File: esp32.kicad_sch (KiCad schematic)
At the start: 13 parts, among them J2 Conn_01x05_Pin, Q3 MMBT3904, Q4 MMBT3904, U14 S32K324NHT1MPBST, Y1 ECS-2520MV-xxx-xx

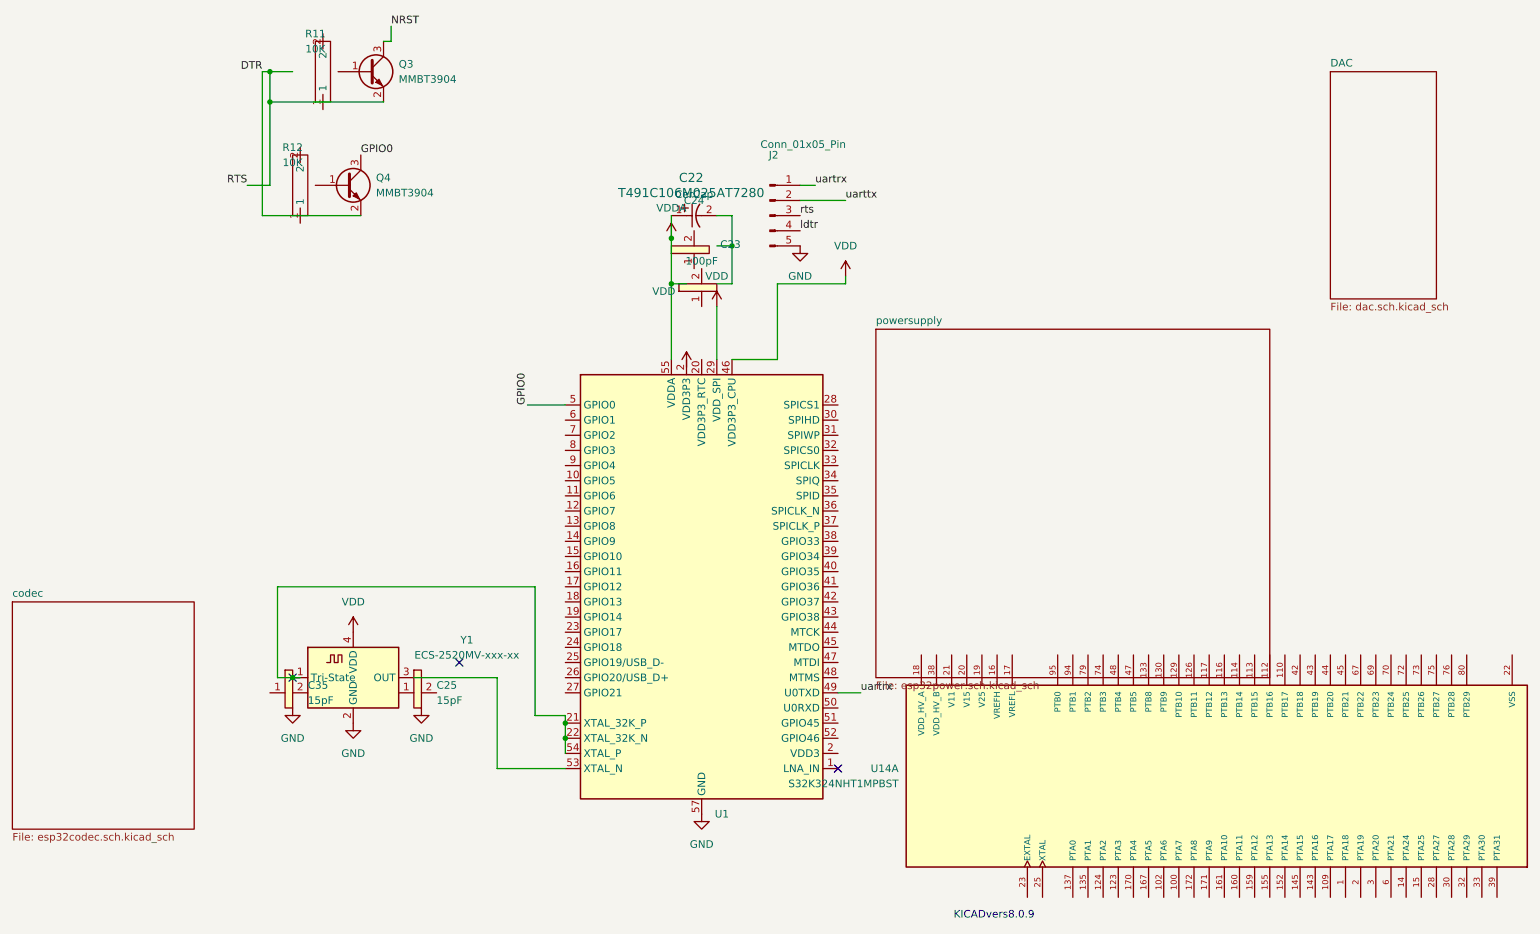
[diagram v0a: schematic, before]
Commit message: recloned first commit
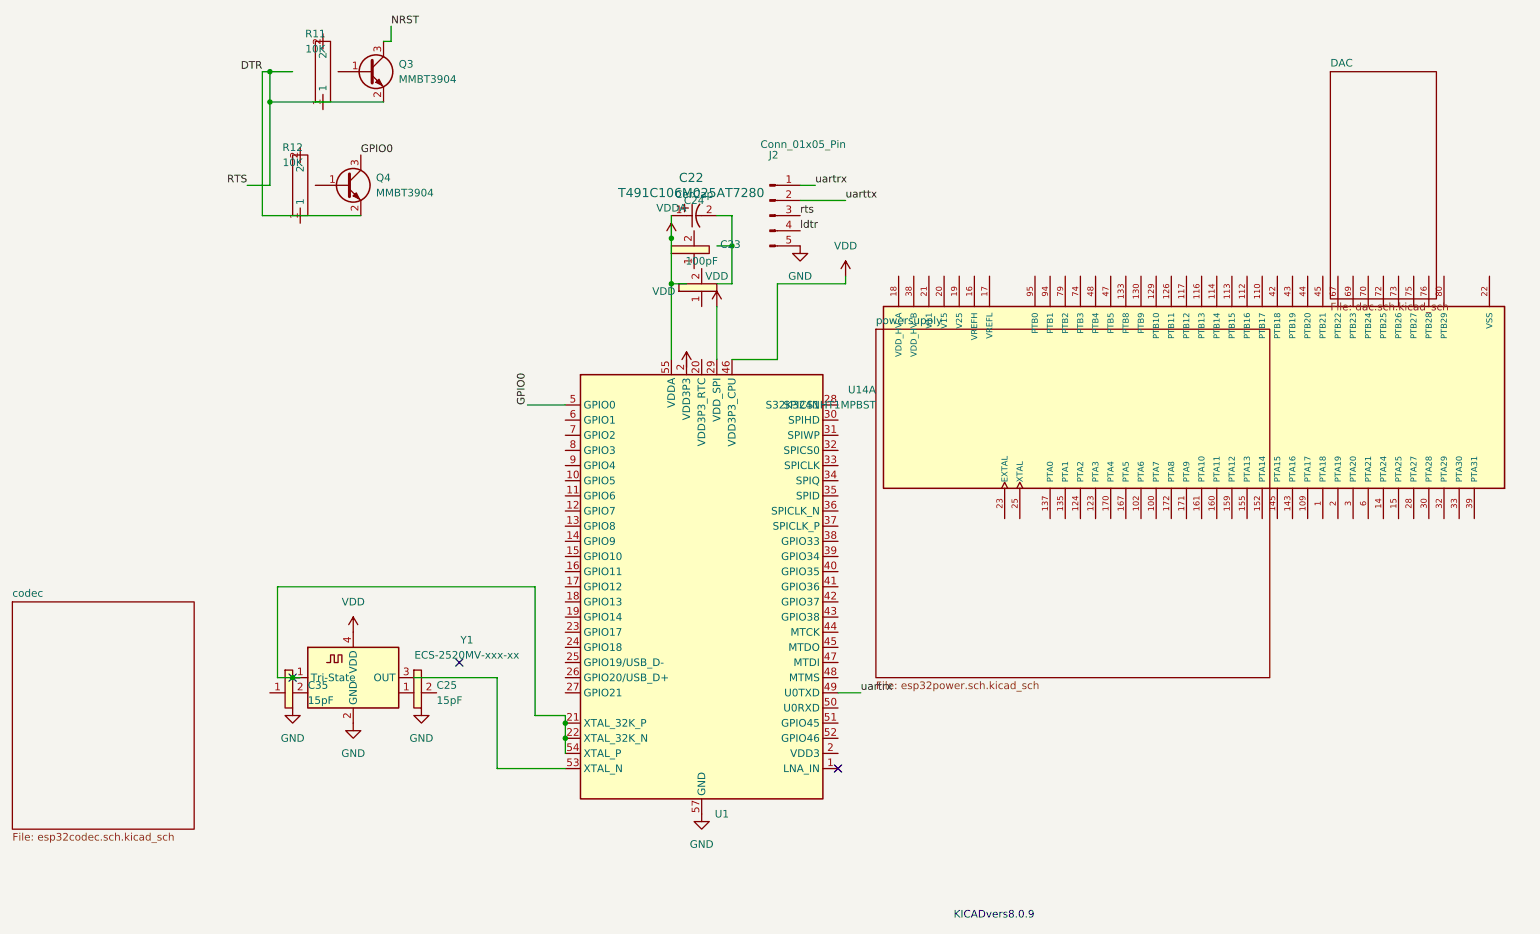
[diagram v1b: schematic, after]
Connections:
- net at U1.2 (VDD3P3): now also U1.3 (VDD3P3)
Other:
- moved on the sheet: U14A
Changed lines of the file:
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@@
 	(symbol
 		(lib_id "common:S32K324NHT1MPBST")
-		(at 226.06 148.59 90)
+		(at 222.25 85.09 90)
 		(unit 1)
 		(exclude_from_sim no)
@@
 		(fields_autoplaced yes)
 		(property "Reference" "U14"
-			(at 171.45 147.3199 90)
+			(at 167.64 83.8199 90)
 			(effects
 				(font
@@
 		)
 		(property "Value" "S32K324NHT1MPBST"
-			(at 171.45 149.8599 90)
+			(at 167.64 86.3599 90)
 			(effects
 				(font
@@
 		)
 		(property "Footprint" "commonfootprint:IC_S32K324NHT1MPBST"
-			(at 226.06 148.59 0)
+			(at 222.25 85.09 0)
 			(effects
 				(font
@@
 		)
 		(property "Datasheet" ""
-			(at 226.06 148.59 0)
+			(at 222.25 85.09 0)
 			(effects
 				(font
@@
 		)
 		(property "Description" ""
-			(at 226.06 148.59 0)
+			(at 222.25 85.09 0)
 			(effects
 				(font
@@
 		)
 		(property "MF" "NXP Semiconductors"
-			(at 226.06 148.59 0)
+			(at 222.25 85.09 0)
 			(effects
 				(font
@@
 		)
 		(property "MAXIMUM_PACKAGE_HEIGHT" "1.65 mm"
-			(at 226.06 148.59 0)
+			(at 222.25 85.09 0)
 			(effects
 				(font
@@
 		)
 		(property "Package" "QFP-172 NXP"
-			(at 226.06 148.59 0)
+			(at 222.25 85.09 0)
 			(effects
 				(font
@@
 		)
 		(property "Price" "None"
-			(at 226.06 148.59 0)
+			(at 222.25 85.09 0)
 			(effects
 				(font
@@
 		)
 		(property "Check_prices" "https://www.snapeda.com/parts/S32K324NHT1MPBST/NXP+Semiconductors/view-part/?ref=eda"
-			(at 226.06 148.59 0)
+			(at 222.25 85.09 0)
 			(effects
 				(font
@@
 		)
 		(property "STANDARD" "Manufacturer Recommendations"
-			(at 226.06 148.59 0)
+			(at 222.25 85.09 0)
 			(effects
 				(font
@@
 		)
 		(property "PARTREV" "7"
-			(at 226.06 148.59 0)
+			(at 222.25 85.09 0)
 			(effects
 				(font
@@
 		)
 		(property "SnapEDA_Link" "https://www.snapeda.com/parts/S32K324NHT1MPBST/NXP+Semiconductors/view-part/?ref=snap"
-			(at 226.06 148.59 0)
+			(at 222.25 85.09 0)
 			(effects
 				(font
@@
 		)
 		(property "MP" "S32K324NHT1MPBST"
-			(at 226.06 148.59 0)
+			(at 222.25 85.09 0)
 			(effects
 				(font
@@
 		)
 		(property "Description_1" "\n                        \n                            ARM® Cortex®-M7 Automotive, AEC-Q100, S32K3 Microcontroller IC 32-Bit Dual-Core 160MHz 4MB (4M x 8) FLASH 172-QFP (16x16)\n                        \n"
-			(at 226.06 148.59 0)
+			(at 222.25 85.09 0)
 			(effects
 				(font
@@
 		)
 		(property "SNAPEDA_PN" "121580"
-			(at 226.06 148.59 0)
+			(at 222.25 85.09 0)
 			(effects
 				(font
@@
 		)
 		(property "Availability" "In Stock"
-			(at 226.06 148.59 0)
+			(at 222.25 85.09 0)
 			(effects
 				(font
@@
 		)
 		(property "MANUFACTURER" "NXP Semiconductors"
-			(at 226.06 148.59 0)
+			(at 222.25 85.09 0)
 			(effects
 				(font
